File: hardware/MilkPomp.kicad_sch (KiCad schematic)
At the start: 13 parts, among them J1 Screw_Terminal_01x06, J4 Conn_Board, J5 Conn_Display, J6 PWR INPUT

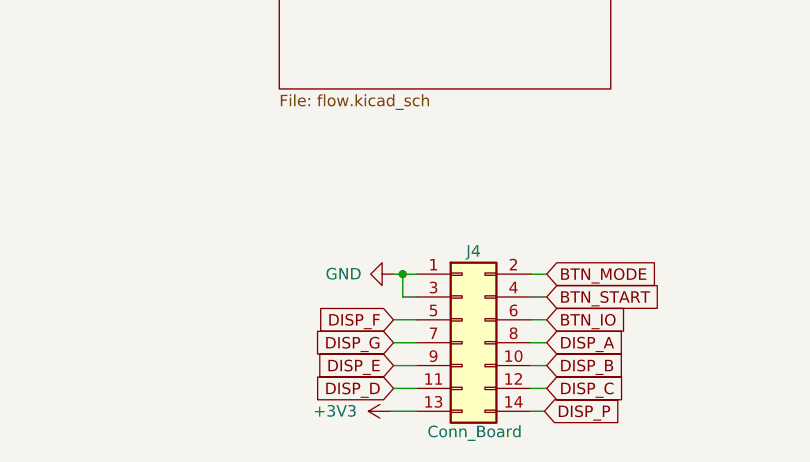
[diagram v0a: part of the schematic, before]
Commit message: PCB design completed
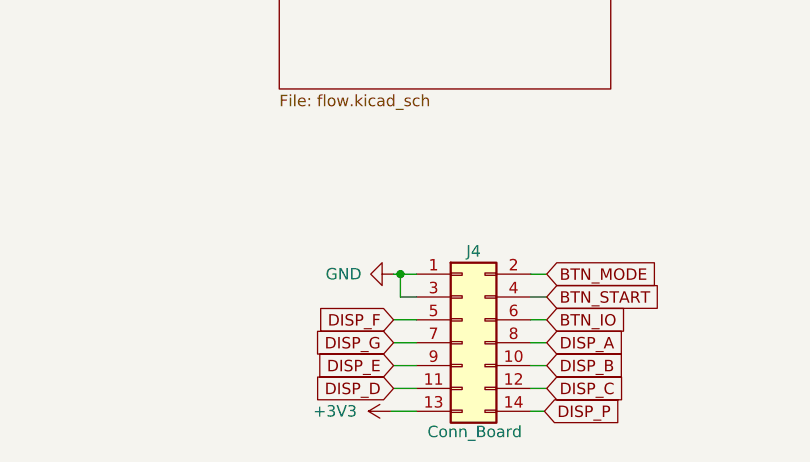
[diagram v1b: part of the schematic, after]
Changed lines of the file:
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@@
   (junction (at 37.846 100.33) (diameter 0) (color 0 0 0 0)
   )
-  (junction (at 134.366 168.656) (diameter 0) (color 0 0 0 0)
+  (junction (at 134.112 168.656) (diameter 0) (color 0 0 0 0)
   )
   (wire (pts (xy 65.024 81.534) (xy 67.818 81.534))
@@
     (stroke (width 0) (type default) (color 0 0 0 0))
   )
+  (wire (pts (xy 134.112 171.196) (xy 134.112 168.656))
+    (stroke (width 0) (type default) (color 0 0 0 0))
+  )
   (wire (pts (xy 148.59 178.816) (xy 150.368 178.816))
     (stroke (width 0) (type default) (color 0 0 0 0))
   )
   (wire (pts (xy 36.576 100.33) (xy 37.846 100.33))
-    (stroke (width 0) (type default) (color 0 0 0 0))
-  )
-  (wire (pts (xy 135.89 171.196) (xy 134.366 171.196))
     (stroke (width 0) (type default) (color 0 0 0 0))
   )
@@
   )
   (wire (pts (xy 157.48 133.604) (xy 202.946 133.604))
-    (stroke (width 0) (type default) (color 0 0 0 0))
-  )
-  (wire (pts (xy 134.366 168.656) (xy 134.366 171.196))
     (stroke (width 0) (type default) (color 0 0 0 0))
   )
@@
     (stroke (width 0) (type default) (color 0 0 0 0))
   )
-  (wire (pts (xy 133.35 168.656) (xy 134.366 168.656))
-    (stroke (width 0) (type default) (color 0 0 0 0))
-  )
   (polyline (pts (xy 283.21 13.716) (xy 283.21 56.007))
     (stroke (width 0) (type default) (color 0 0 0 0))
@@
     (stroke (width 0) (type default) (color 0 0 0 0))
   )
+  (wire (pts (xy 135.89 171.196) (xy 134.112 171.196))
+    (stroke (width 0) (type default) (color 0 0 0 0))
+  )
   (wire (pts (xy 202.946 101.346) (xy 202.946 122.682))
+    (stroke (width 0) (type default) (color 0 0 0 0))
+  )
+  (wire (pts (xy 133.35 168.656) (xy 134.112 168.656))
     (stroke (width 0) (type default) (color 0 0 0 0))
   )
@@
   )
   (wire (pts (xy 68.072 50.8) (xy 62.738 50.8))
-    (stroke (width 0) (type default) (color 0 0 0 0))
-  )
-  (wire (pts (xy 134.366 168.656) (xy 135.89 168.656))
     (stroke (width 0) (type default) (color 0 0 0 0))
   )
@@
     (stroke (width 0) (type default) (color 0 0 0 0))
   )
+  (wire (pts (xy 134.112 168.656) (xy 135.89 168.656))
+    (stroke (width 0) (type default) (color 0 0 0 0))
+  )
